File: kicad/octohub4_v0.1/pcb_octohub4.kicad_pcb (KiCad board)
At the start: 2 copper layers, 100 x 80 mm, 85 parts, among them J101 USB231ARY, J102 USB231ARY, J103 USB231ARY, J104 USB231ARY, J201 Screw_Terminal_01x02, J203 Barrel_Jack_Switch, J301 USB_C_Receptacle_USB2.0, U201 TPS259474LRPWR, U301 AMS1117-3.3, U302 USB2514B_Bi, Y301 24MHz

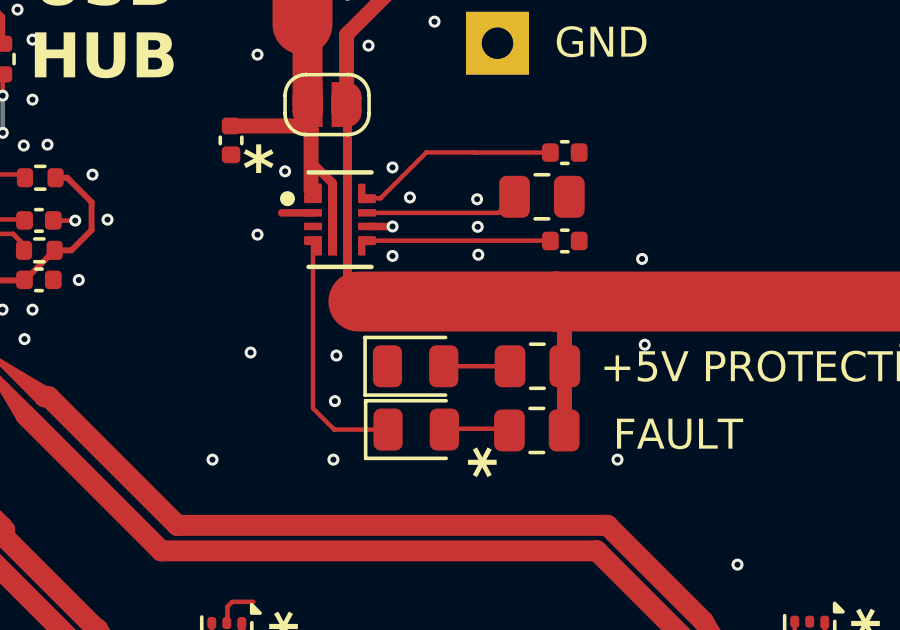
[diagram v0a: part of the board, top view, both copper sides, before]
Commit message: Version v0.1
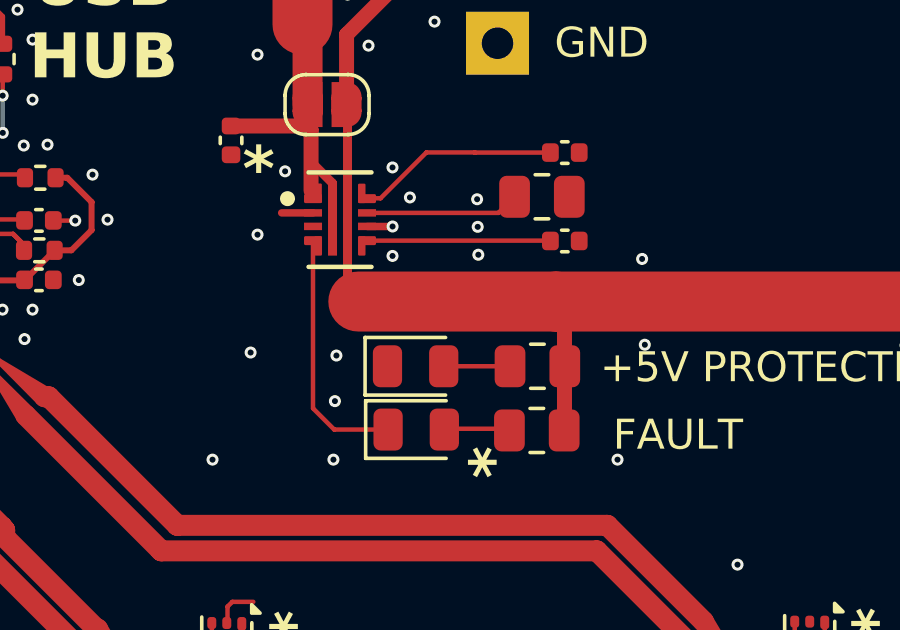
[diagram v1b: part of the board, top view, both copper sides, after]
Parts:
- R201: value 120 -> 680
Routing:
- net +5VIN: track 256.6 -> 255.9 mm
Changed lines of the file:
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@@
 			)
 		)
-		(property "KiCadOriginal" "MountingHole_3.2mm_M3_DIN965_Pad"
-			(at 0 0 0)
-			(layer "F.SilkS")
-			(hide yes)
-			(effects
-				(font
-					(size 1 1)
-					(thickness 0.1)
-				)
-			)
-		)
 		(property ki_fp_filters "MountingHole*Pad*")
 		(sheetname "/Power Protection/")
@@
 			)
 		)
-		(property "KiCadOriginal" "MountingHole_3.2mm_M3_DIN965_Pad"
-			(at 0 0 0)
-			(layer "F.SilkS")
-			(hide yes)
-			(effects
-				(font
-					(size 1 1)
-					(thickness 0.1)
-				)
-			)
-		)
 		(property ki_fp_filters "MountingHole*Pad*")
 		(sheetname "/Power Protection/")
@@
 			)
 		)
-		(property "KiCadOriginal" "TerminalBlock_WAGO_236-402_1x02_P5.00mm_45Degree"
-			(at 0 0 90)
-			(layer "F.SilkS")
-			(hide yes)
-			(effects
-				(font
-					(size 1 1)
-					(thickness 0.1)
-				)
-			)
-		)
 		(property ki_fp_filters "TerminalBlock*:*")
 		(sheetname "/Power Protection/")
@@
 			)
 		)
-		(property "KiCadOrigin" "BarrelJack_CUI_PJ-079BH_Horizontal"
-			(at 0 0 90)
-			(layer "F.SilkS")
-			(hide yes)
-			(effects
-				(font
-					(size 1 1)
-					(thickness 0.1)
-				)
-			)
-		)
 		(property "JLCPCB" "C319095"
 			(at 0 0 270)
@@
 			)
 		)
-		(property "Value" "120"
+		(property "Value" "680"
 			(at 0 1.65 0)
 			(layer "F.Fab")
@@
 			)
 		)
-		(property "KiCadOriginal" "MountingHole_3.2mm_M3_DIN965_Pad"
-			(at 0 0 0)
-			(layer "F.SilkS")
-			(hide yes)
-			(effects
-				(font
-					(size 1 1)
-					(thickness 0.1)
-				)
-			)
-		)
 		(property ki_fp_filters "MountingHole*Pad*")
 		(sheetname "/Power Protection/")
@@
 			)
 		)
-		(property "KiCadOriginal" "MountingHole_3.2mm_M3_DIN965_Pad"
-			(at 0 0 0)
-			(layer "F.SilkS")
-			(hide yes)
-			(effects
-				(font
-					(size 1 1)
-					(thickness 0.1)
-				)
-			)
-		)
 		(property ki_fp_filters "MountingHole*Pad*")
 		(sheetname "/Power Protection/")
@@
 	)
 	(segment
-		(start 124.26 65.99)
-		(end 124.26 66.4)
-		(width 0.3)
-		(layer "F.Cu")
-		(net 1)
-	)
-	(segment
 		(start 123.4432 63.6612)
 		(end 123.5448 63.7628)
@@
 	)
 	(segment
-		(start 124.26 66.4)
-		(end 124.26 66.76)
-		(width 0.3)
-		(layer "F.Cu")
-		(net 1)
-	)
-	(segment
 		(start 72.41 23.26)
 		(end 73.76 23.26)
@@
 		(layer "F.Cu")
 		(net 2)
-	)
-	(segment
-		(start 131.9825 73.7875)
-		(end 131.9925 73.7775)
-		(width 0.5)
-		(layer "F.Cu")
-		(net 2)
